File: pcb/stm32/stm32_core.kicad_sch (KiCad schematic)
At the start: 1 part

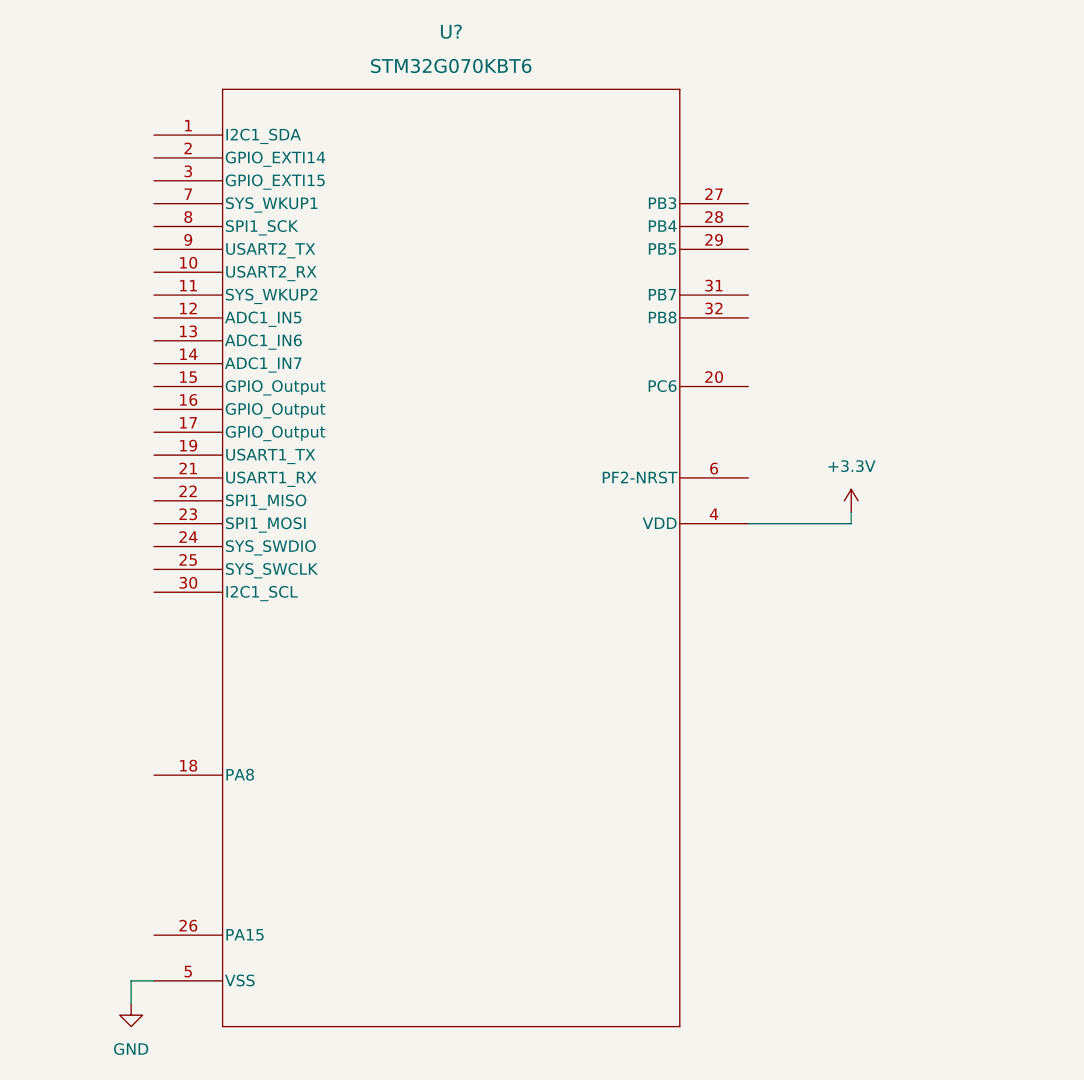
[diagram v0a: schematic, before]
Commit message: Fixed schema
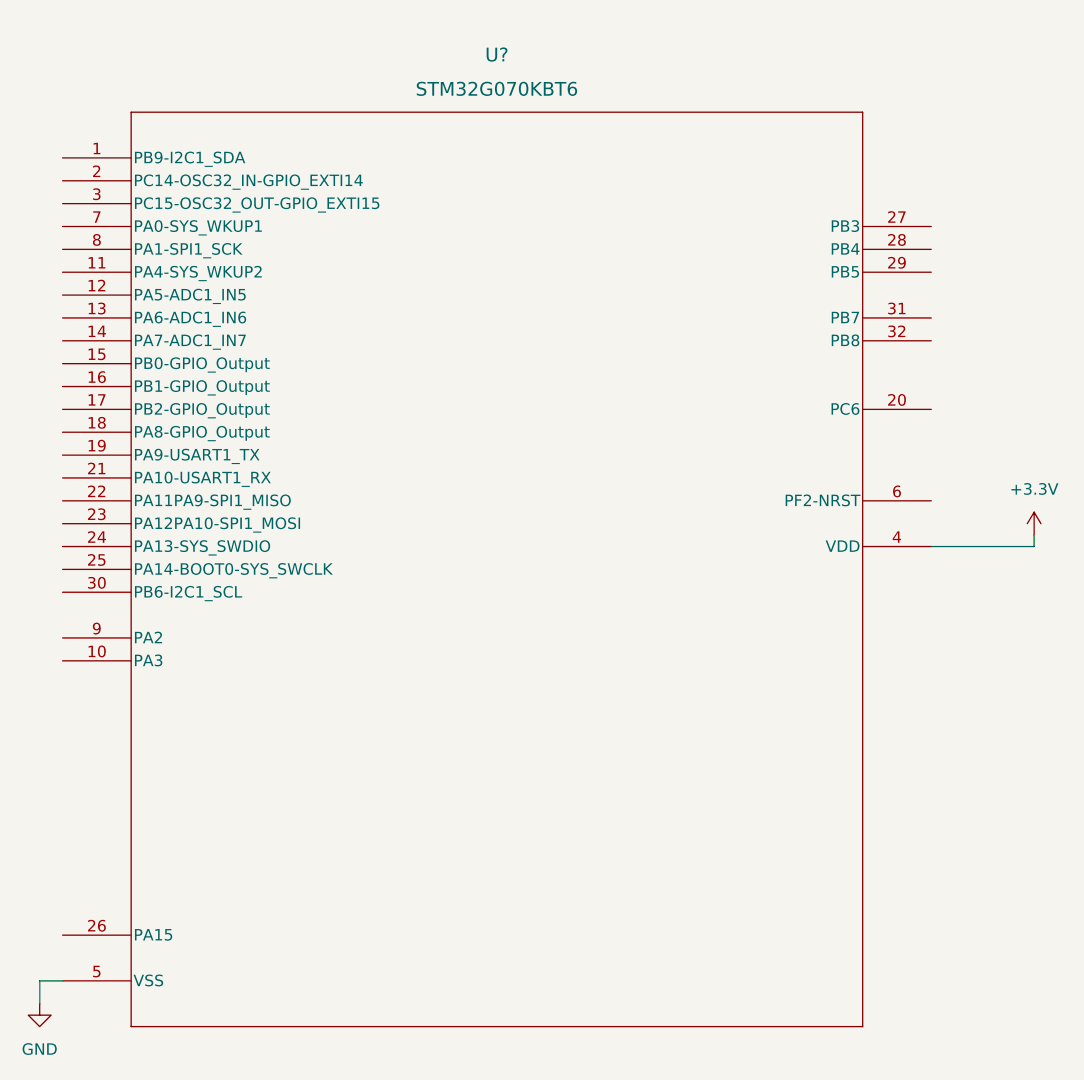
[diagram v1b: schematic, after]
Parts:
- removed U?: STM32G070KBT6, LQFP-32, symbol 2023-02-12_17-09-08:STM32G070KBT6
- added U?: STM32G070KBT6, LQFP-32, symbol 2023-02-13_13-40-03:STM32G070KBT6
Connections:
- net +3.3V: now also U?.4 (VDD)
- net GND: now also U?.5 (VSS)
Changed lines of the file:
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@@
 (kicad_sch (version 20211123) (generator eeschema)
   (paper "A4")
-  (wire (pts (xy 190.5 90.17) (xy 190.5 88.9))
+  (wire (pts (xy 210.82 92.71) (xy 210.82 91.44))
     (stroke (width 0) (type default) (color 0 0 0 0))
   )
-  (wire (pts (xy 110.49 143.51) (xy 110.49 140.97))
+  (wire (pts (xy 100.33 143.51) (xy 100.33 140.97))
     (stroke (width 0) (type default) (color 0 0 0 0))
   )
-  (wire (pts (xy 110.49 140.97) (xy 113.03 140.97))
+  (wire (pts (xy 100.33 140.97) (xy 102.87 140.97))
     (stroke (width 0) (type default) (color 0 0 0 0))
   )
-  (wire (pts (xy 179.07 90.17) (xy 190.5 90.17))
+  (wire (pts (xy 199.39 92.71) (xy 210.82 92.71))
     (stroke (width 0) (type default) (color 0 0 0 0))
   )
-  (symbol (lib_id "power:GND") (at 110.49 143.51 0) (unit 1)
+  (symbol (lib_id "2023-02-13_13-40-03:STM32G070KBT6") (at 102.87 49.53 0) (unit 1)
     (in_bom yes) (on_board yes) (fields_autoplaced)
-    (property "Reference" "#PWR?" (id 0) (at 110.49 149.86 0)
-      (effects (font (size 1.27 1.27)) hide)
-    )
-    (property "Value" "GND" (id 1) (at 110.49 148.59 0))
-    (property "Footprint" "" (id 2) (at 110.49 143.51 0)
-      (effects (font (size 1.27 1.27)) hide)
-    )
-    (property "Datasheet" "" (id 3) (at 110.49 143.51 0)
-      (effects (font (size 1.27 1.27)) hide)
-    )
-    (pin "1")
-  )
-  (symbol (lib_id "2023-02-12_17-09-08:STM32G070KBT6") (at 113.03 46.99 0) (unit 1)
-    (in_bom yes) (on_board yes) (fields_autoplaced)
-    (property "Reference" "U?" (id 0) (at 146.05 35.56 0)
+    (property "Reference" "U?" (id 0) (at 151.13 38.1 0)
       (effects (font (size 1.524 1.524)))
     )
-    (property "Value" "STM32G070KBT6" (id 1) (at 146.05 39.37 0)
+    (property "Value" "STM32G070KBT6" (id 1) (at 151.13 41.91 0)
       (effects (font (size 1.524 1.524)))
     )
-    (property "Footprint" "LQFP-32" (id 2) (at 113.03 46.99 0)
+    (property "Footprint" "LQFP-32" (id 2) (at 102.87 49.53 0)
       (effects (font (size 1.27 1.27) italic) hide)
     )
-    (property "Datasheet" "STM32G070KBT6" (id 3) (at 113.03 46.99 0)
+    (property "Datasheet" "STM32G070KBT6" (id 3) (at 102.87 49.53 0)
       (effects (font (size 1.27 1.27) italic) hide)
     )
@@
     (pin "9")
   )
-  (symbol (lib_id "power:+3.3V") (at 190.5 88.9 0) (unit 1)
+  (symbol (lib_id "power:GND") (at 100.33 143.51 0) (unit 1)
     (in_bom yes) (on_board yes) (fields_autoplaced)
-    (property "Reference" "#PWR?" (id 0) (at 190.5 92.71 0)
+    (property "Reference" "#PWR?" (id 0) (at 100.33 149.86 0)
       (effects (font (size 1.27 1.27)) hide)
     )
-    (property "Value" "+3.3V" (id 1) (at 190.5 83.82 0))
-    (property "Footprint" "" (id 2) (at 190.5 88.9 0)
+    (property "Value" "GND" (id 1) (at 100.33 148.59 0))
+    (property "Footprint" "" (id 2) (at 100.33 143.51 0)
       (effects (font (size 1.27 1.27)) hide)
     )
-    (property "Datasheet" "" (id 3) (at 190.5 88.9 0)
+    (property "Datasheet" "" (id 3) (at 100.33 143.51 0)
       (effects (font (size 1.27 1.27)) hide)
     )
+    (pin "1")
+  )
+  (symbol (lib_id "power:+3.3V") (at 210.82 91.44 0) (unit 1)
+    (in_bom yes) (on_board yes) (fields_autoplaced)
+    (property "Reference" "#PWR?" (id 0) (at 210.82 95.25 0)
+      (effects (font (size 1.27 1.27)) hide)
+    )
+    (property "Value" "+3.3V" (id 1) (at 210.82 86.36 0))
+    (property "Footprint" "" (id 2) (at 210.82 91.44 0)
+      (effects (font (size 1.27 1.27)) hide)
+    )
+    (property "Datasheet" "" (id 3) (at 210.82 91.44 0)
+      (effects (font (size 1.27 1.27)) hide)
+    )
